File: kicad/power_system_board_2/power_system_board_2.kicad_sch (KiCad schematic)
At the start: 17 parts, among them J1 USB_C_Receptacle_USB2.0_16P, J2 Conn_01x04_Pin, Q1 NMOS, Q3 PMOS, U1 ${SIM.PARAMS}

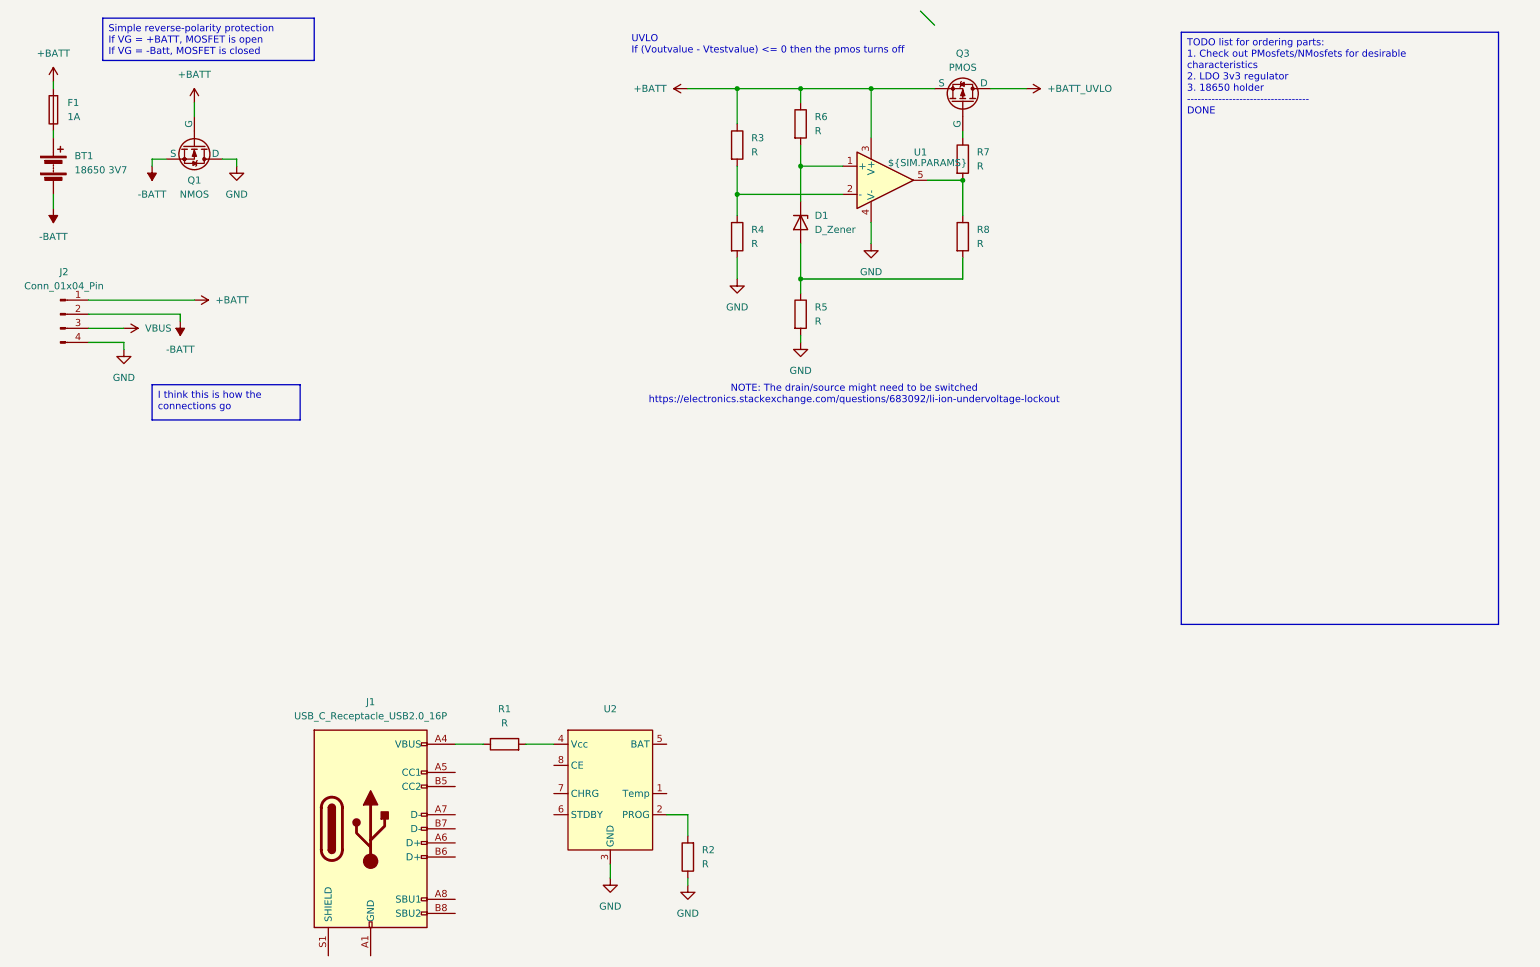
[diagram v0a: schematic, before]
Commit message: Making headway
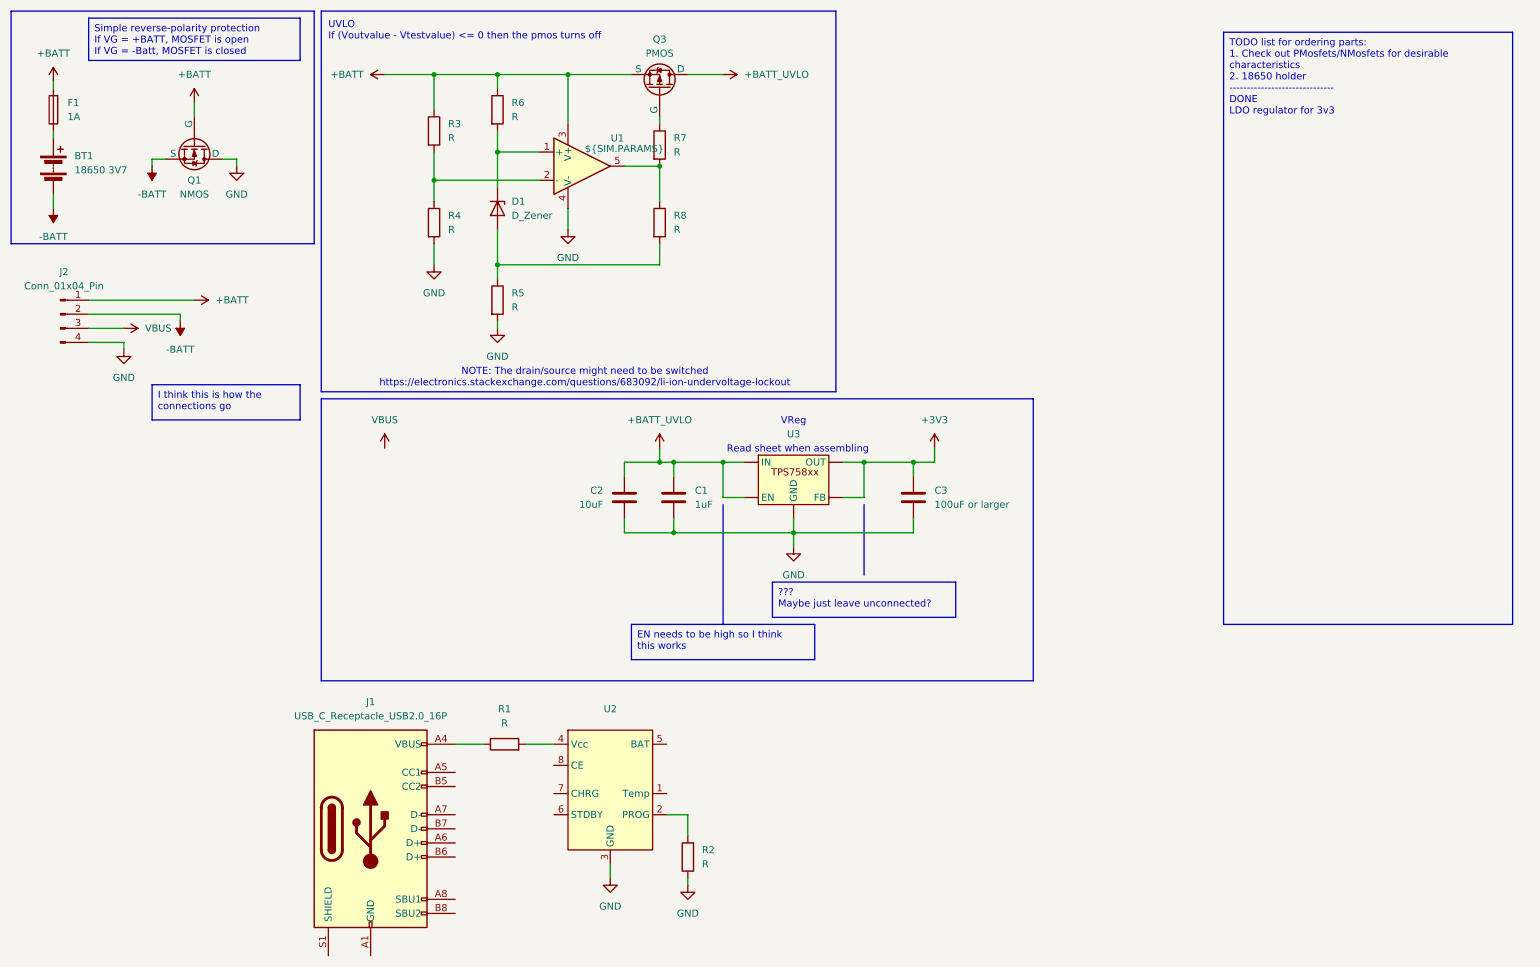
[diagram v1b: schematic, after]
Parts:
- added C1: 1uF, symbol Device:C
- added C2: 10uF, symbol Device:C
- added C3: 100uF or larger, symbol Device:C
- added U3: ~, symbol Custom_Voltage_Regulators:TPS758xx
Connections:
- net +BATT_UVLO: now also C1.1, C2.1, U3. (OUT)
- net GND: now also C1.2, C2.2, C3.2, U3. (OUT)
- new net +3V3: C3.1, U3. (OUT)
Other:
- note added: "Read sheet when assembling"
- note added: "VReg"
- moved on the sheet: D1, Q3, R3, R4, R5, R6, R7, R8, U1
